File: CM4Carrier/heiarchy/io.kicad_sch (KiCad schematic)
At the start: 1 part

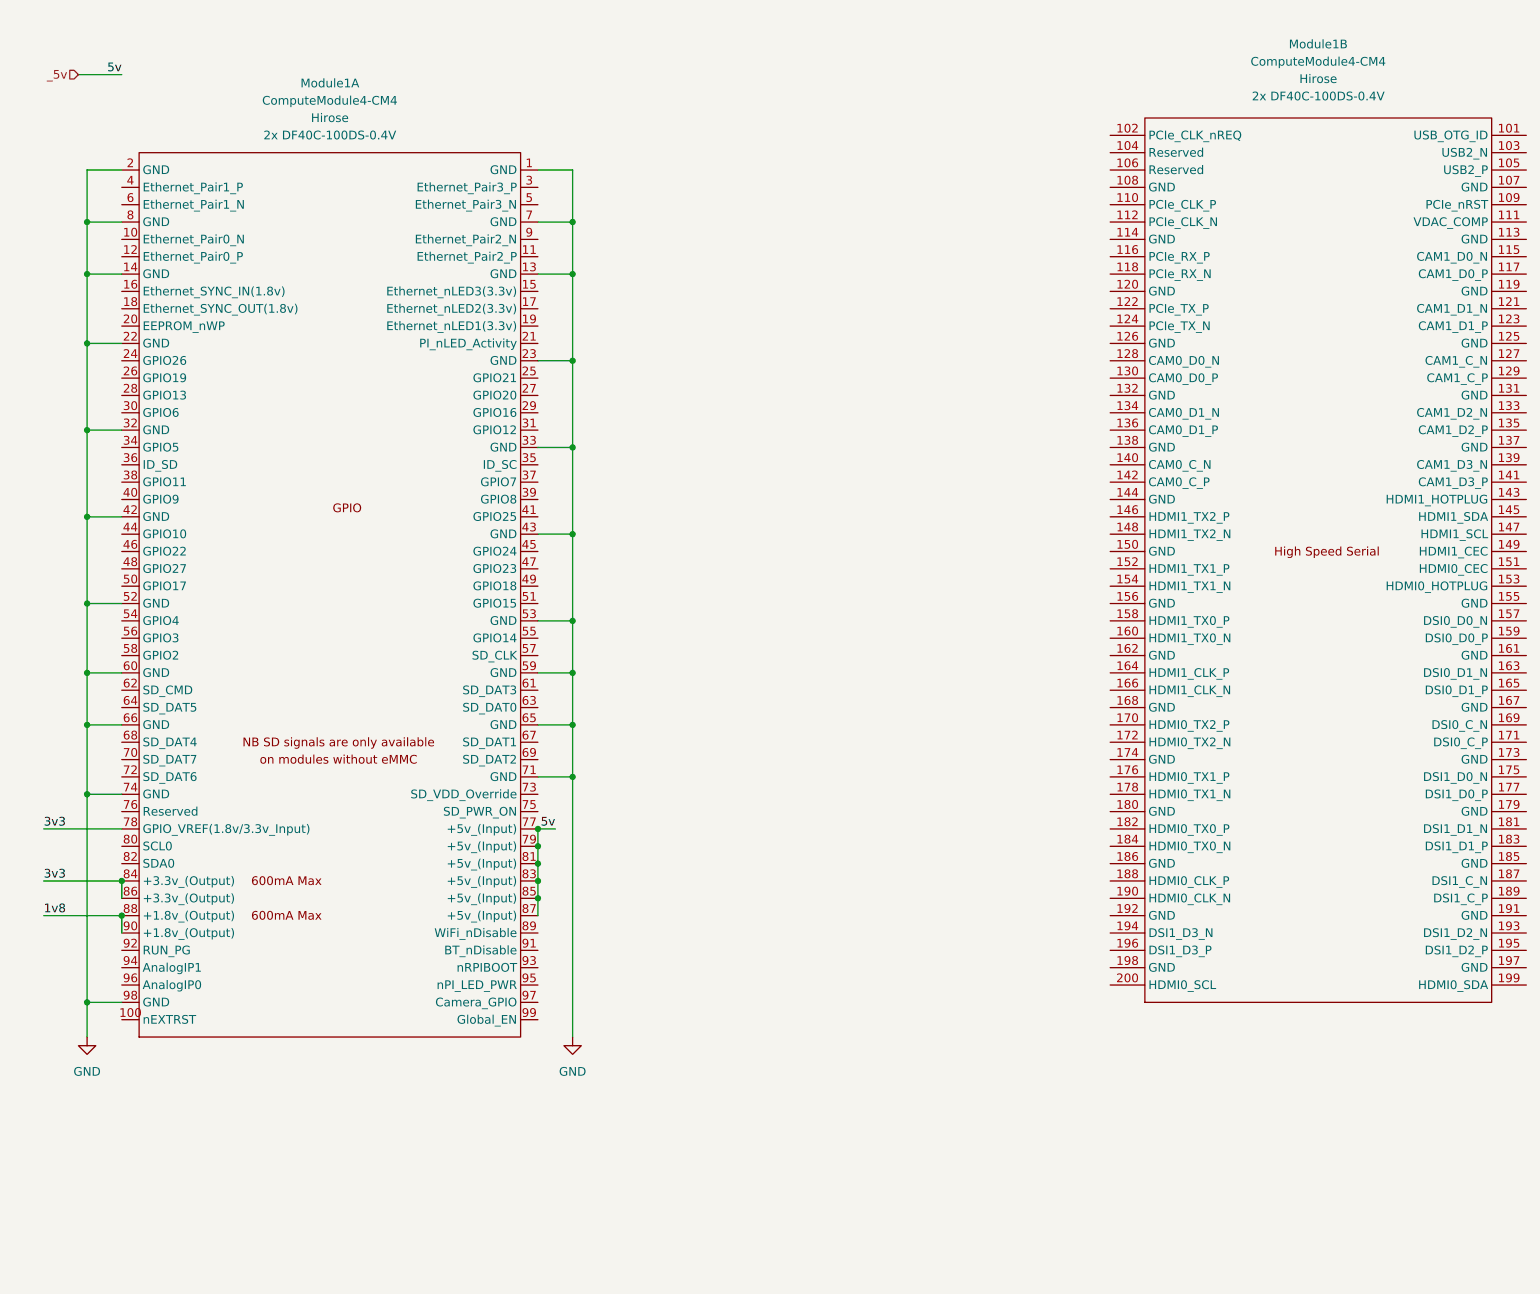
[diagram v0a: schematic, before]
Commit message: aaa
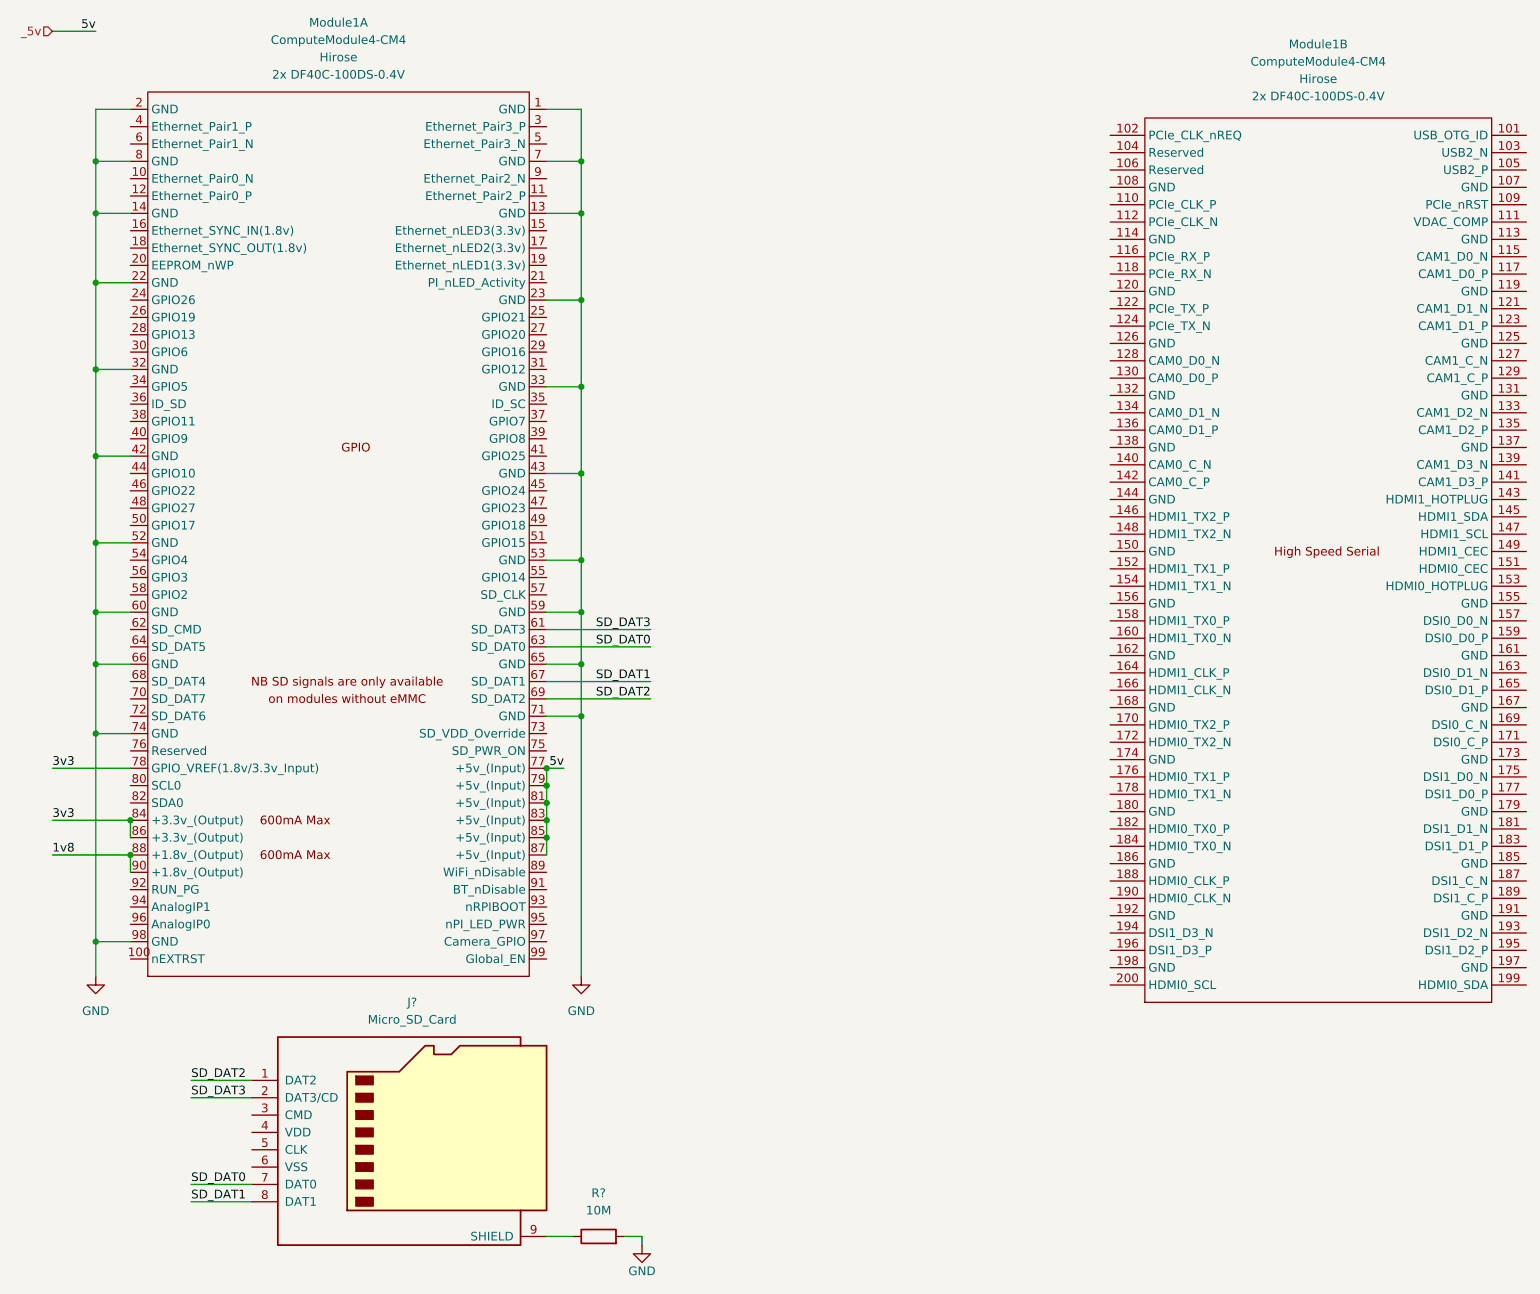
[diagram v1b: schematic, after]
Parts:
- added J?: Micro_SD_Card, symbol Connector:Micro_SD_Card
- added R?: 10M, symbol Device:R
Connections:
- net GND: now also R?.2
- net SD_DAT3: now reaches Module1.61 (SD_DAT3)
- net SD_DAT3: now also J?.2 (DAT3/CD)
- net SD_DAT0: now reaches Module1.63 (SD_DAT0)
- net SD_DAT0: now also J?.7 (DAT0)
- net SD_DAT1: now reaches Module1.67 (SD_DAT1)
- net SD_DAT1: now also J?.8 (DAT1)
- net SD_DAT2: now reaches Module1.69 (SD_DAT2)
- net SD_DAT2: now also J?.1 (DAT2)
- new net: J?.9 (SHIELD), R?.1
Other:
- moved on the sheet: Module1A
